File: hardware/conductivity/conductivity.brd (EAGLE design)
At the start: 32.9 x 35.5 mm, 18 parts, among them IC1 AD820R, U1 TLV2374IDR, U2 TLE2426CD

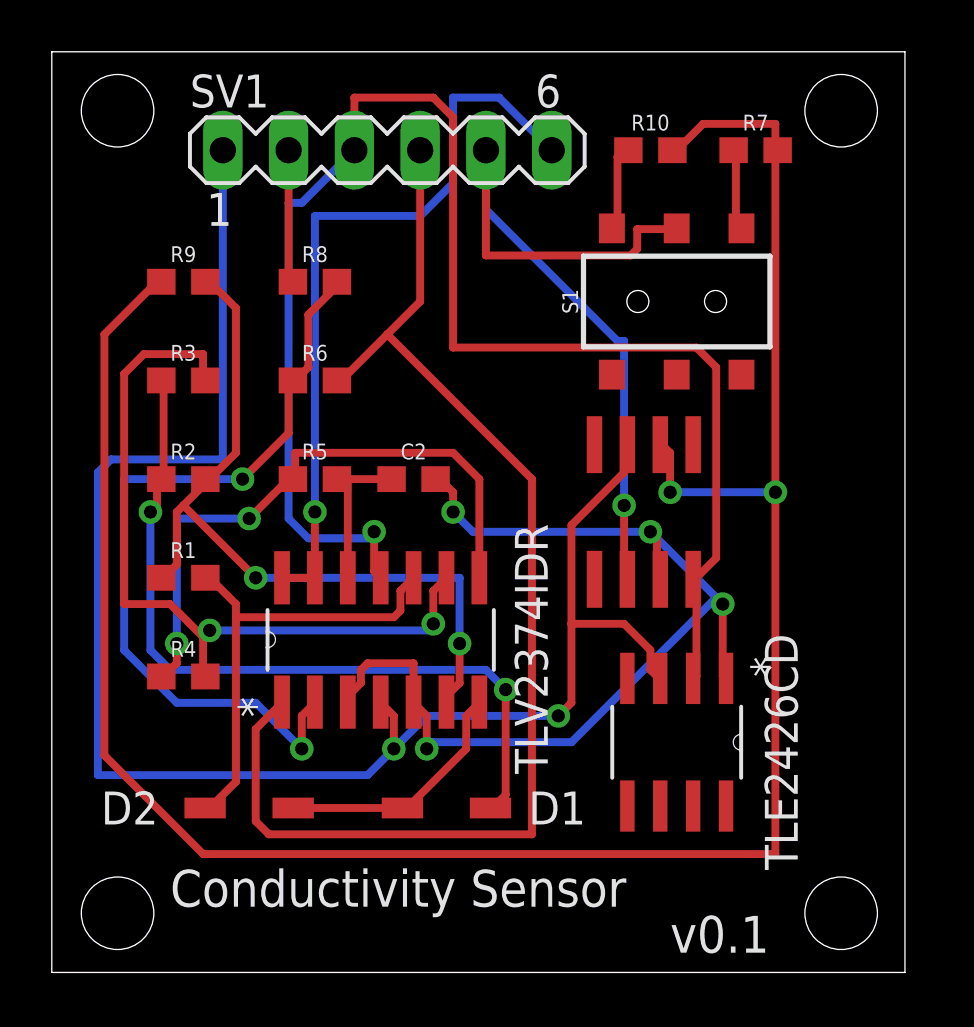
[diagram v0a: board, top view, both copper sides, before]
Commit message: board and parts list update june 2018
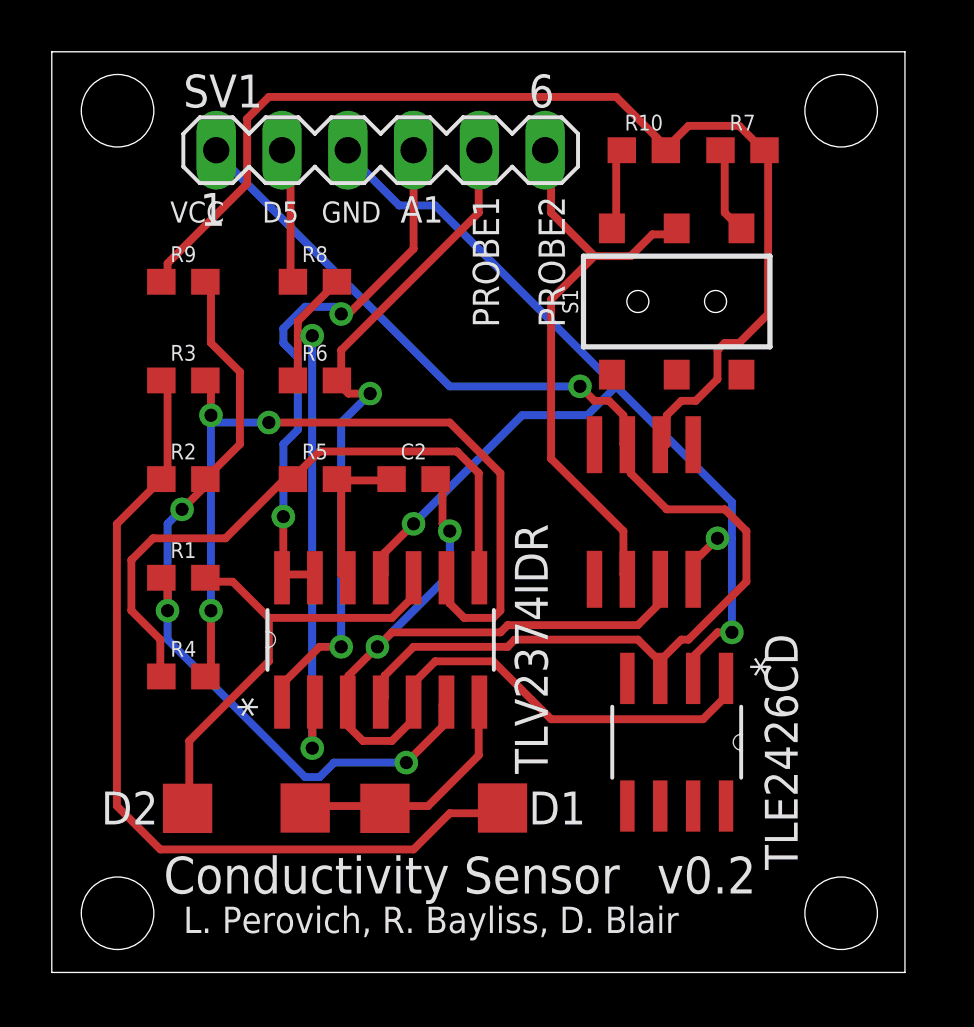
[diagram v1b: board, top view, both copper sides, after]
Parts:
- D1, D2: device fab:SOD123 -> trellisLaura:SOD123
- moved R7 0.51 mm to (26.7, 31.8)
- moved R10 0.25 mm to (22.9, 31.8)
- moved SV1 0.25 mm to (12.7, 31.8)
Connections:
- net FROMWATER: now also SV1.6; no longer SV1.5
- net N$13: now also SV1.4; no longer SV1.6
- net N$16: now also SV1.5; no longer SV1.4
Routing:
- net N$5: track 85.5 -> 43.6 mm, vias 2 -> 0
- net N$16: track 47.8 -> 26.5 mm, vias 0 -> 2
- net N$1: track 65.7 -> 48.3 mm, vias 2 -> 1
- net N$15: track 59.2 -> 43.5 mm, vias 1 -> 3
- net FROMWATER: track 31.3 -> 23.0 mm, vias 1 -> 0
- net N$4: track 31.0 -> 22.9 mm
- net N$13: track 29.1 -> 21.7 mm, vias 1 -> 2
- net N$3: track 39.2 -> 42.9 mm, vias 4 -> 2
- net N$7: track 30.1 -> 33.6 mm, vias 2 -> 0
- net N$10: track 29.6 -> 32.3 mm, vias 2 -> 3
- net N$6: track 30.2 -> 31.9 mm, vias 2 -> 3
- net N$11: track 24.0 -> 24.8 mm, vias 2 -> 0
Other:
- board text added: "A1"
- board text added: "D5"
- board text added: "GND"
- board text added: "L. Perovich, R. Bayliss, D. Blair"
- board text added: "PROBE1"
- board text added: "PROBE2"
- board text added: "VCC"
- board text added: "v0.2"
- board text removed: "v0.1"

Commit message: hardware update
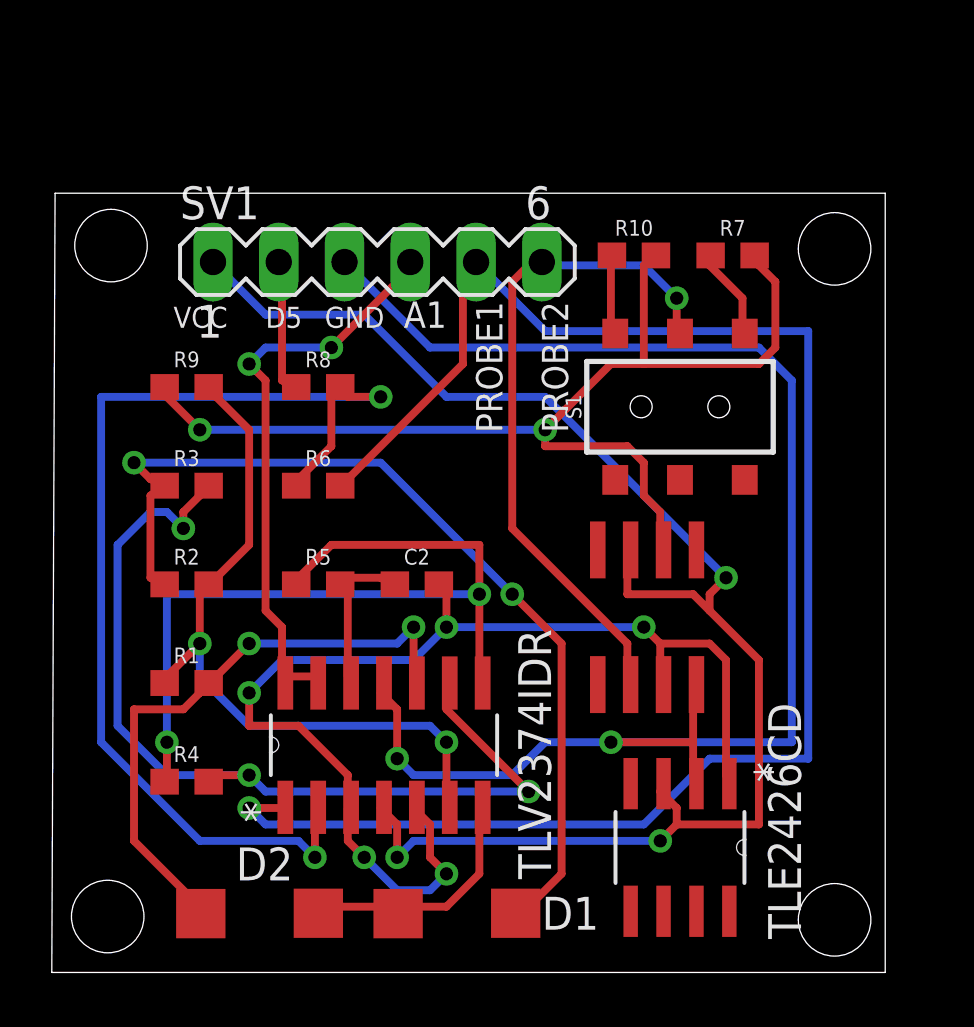
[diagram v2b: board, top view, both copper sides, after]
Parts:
- moved SV1 4.32 mm to (12.6, 27.4)
- moved D1 4.10 mm to (15.7, 2.29)
- moved D2 4.10 mm to (8.13, 2.29)
- moved R10 4.08 mm to (22.5, 27.7)
- moved R7 4.08 mm to (26.3, 27.7)
- moved IC1 4.07 mm to (23.0, 13.7)
- moved U2 4.07 mm to (24.3, 4.83)
- moved C2 4.07 mm to (14.1, 15.0)
- moved R1 4.07 mm to (5.21, 11.2)
- moved R2 4.07 mm to (5.21, 15.0)
- moved R3 4.07 mm to (5.21, 18.8)
- moved R4 4.07 mm to (5.21, 7.37)
- moved R5 4.07 mm to (10.3, 15.0)
- moved R6 4.07 mm to (10.3, 18.8)
- moved R8 4.07 mm to (10.3, 22.6)
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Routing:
- net N$16: track 26.5 -> 65.8 mm, vias 2 -> 1
- net N$4: track 22.9 -> 42.5 mm
- net N$15: track 43.5 -> 59.4 mm, vias 3 -> 2
- net N$1: track 48.3 -> 59.3 mm, vias 1 -> 3
- net N$11: track 24.8 -> 32.5 mm, vias 0 -> 2
- net N$9: track 18.4 -> 23.2 mm, vias 0 -> 2
- net N$10: track 32.3 -> 36.5 mm
- net N$6: track 31.9 -> 27.8 mm, vias 3 -> 2
- net FROMWATER: track 23.0 -> 26.1 mm, vias 0 -> 1
- net N$7: track 33.6 -> 36.6 mm, vias 0 -> 2
- net N$3: track 42.9 -> 44.7 mm, vias 2 -> 5
- net N$5: track 43.6 -> 42.4 mm, vias 0 -> 2
- net N$13: track 21.7 -> 22.6 mm
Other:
- board size 32.9 x 35.5 mm -> 32.2 x 30.1 mm
